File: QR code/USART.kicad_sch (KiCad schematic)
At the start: 26 parts, among them J1 ON_24, J5 ON_5_3, J7 Usart_debbag, U4 AM1SS-2403SJZ, U4 AM1SS-2405SJZ, U5 Pai122E30

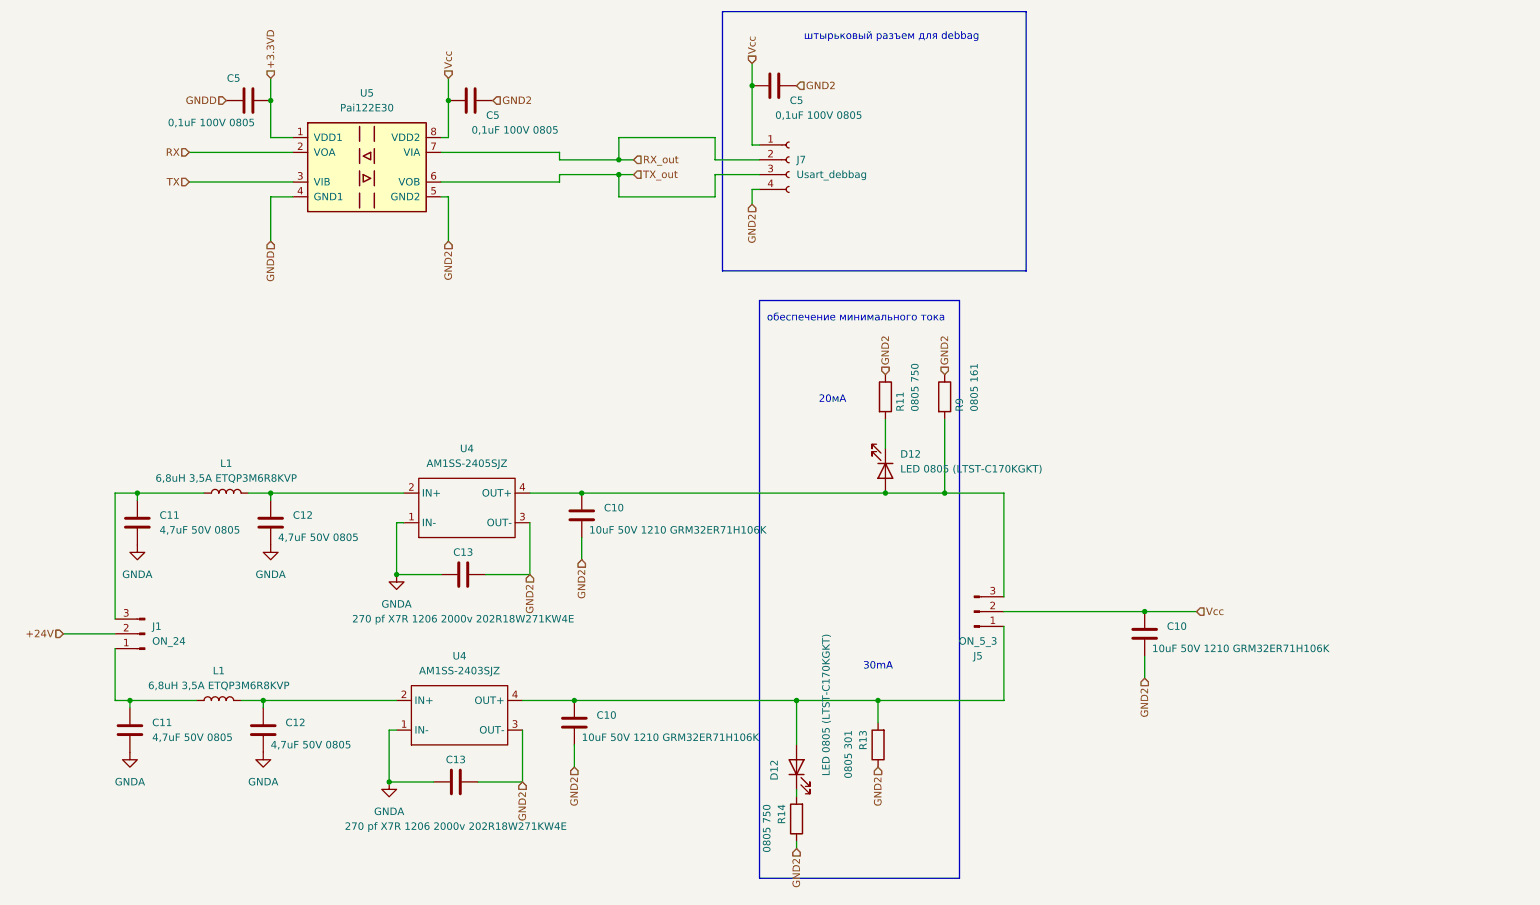
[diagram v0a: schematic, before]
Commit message: qr code schems
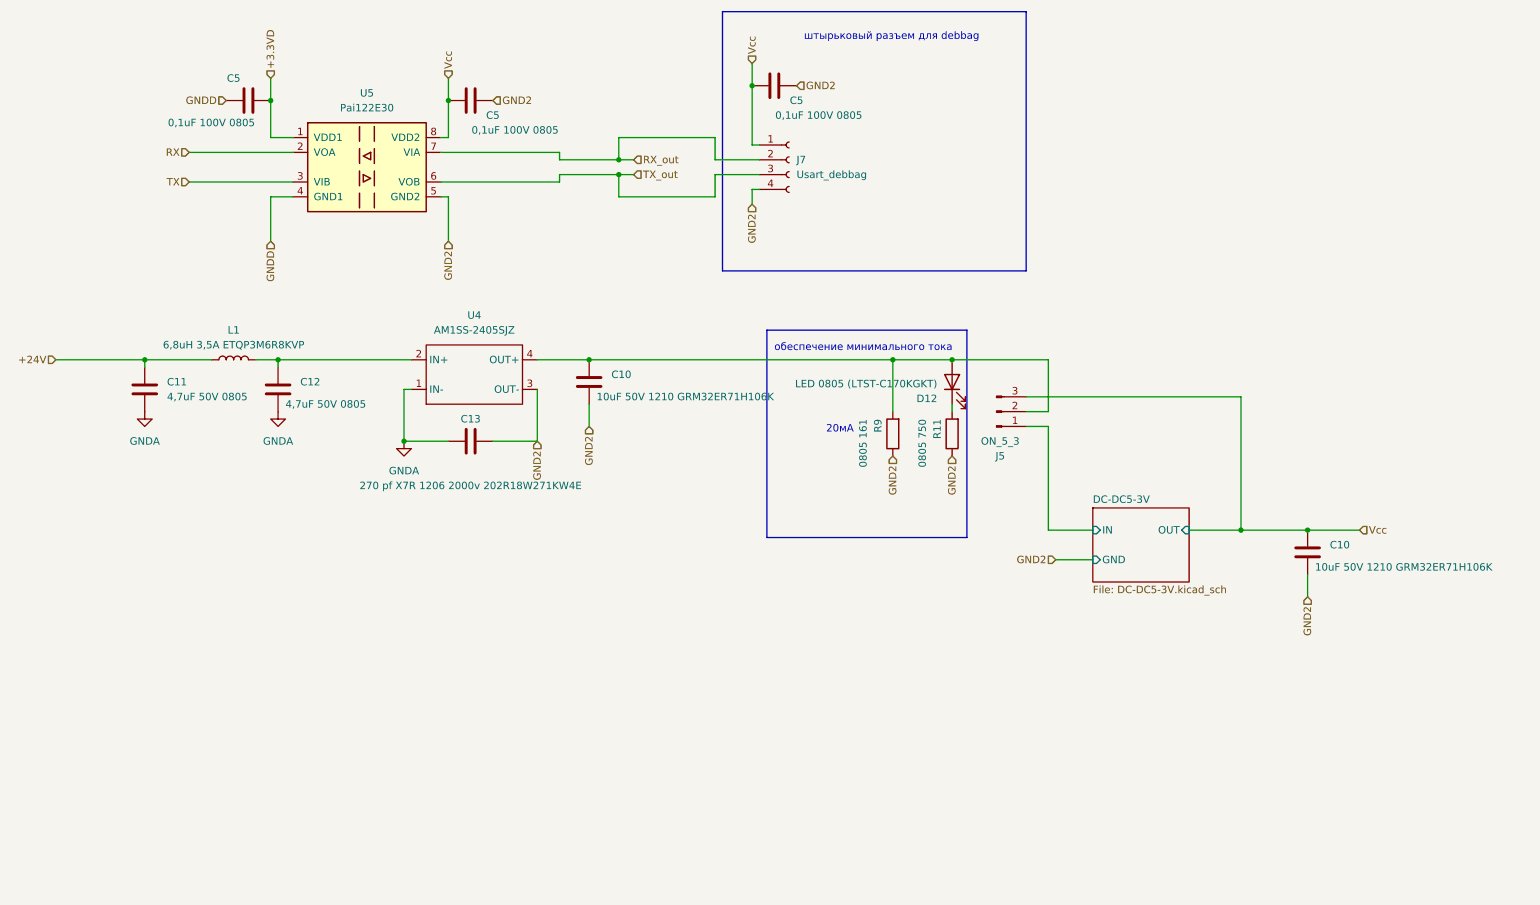
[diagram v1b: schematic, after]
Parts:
- removed C10: 10uF 50V 1210 GRM32ER71H106K, PCM_Capacitor_SMD_AKL:C_1210_3225Metric_Pad1.42x2.65mm_HandSolder, symbol Device:C
- removed C11, C12: 4,7uF 50V 0805, PCM_Capacitor_SMD_AKL:C_0805_2012Metric_Pad1.18x1.45mm_HandSolder, symbol Device:C
- removed C13: 270 pf X7R 1206 2000v 202R18W271KW4E, PCM_Capacitor_SMD_Handsoldering_AKL:C_1210_3225Metric_Pad1.42x2.65mm, symbol Device:C
- removed D12: LED 0805 (LTST-C170KGKT), LED_SMD:LED_0805_2012Metric_Pad1.15x1.40mm_HandSolder, symbol Device:LED
- removed J1: ON_24, Connector_PinHeader_2.54mm:PinHeader_1x03_P2.54mm_Vertical, symbol Connector:Conn_01x03_Pin
- removed L1: 6,8uH 3,5A ETQP3M6R8KVP, PCM_Inductor_SMD_Handsoldering_AKL:L_Bourns-SRN6028, symbol Device:L
- removed R13: 0805 301, Resistor_SMD:R_0805_2012Metric_Pad1.20x1.40mm_HandSolder, symbol Device:R
- removed R14: 0805 750, Resistor_SMD:R_0805_2012Metric_Pad1.20x1.40mm_HandSolder, symbol Device:R
- removed U4: AM1SS-2403SJZ, Converter_DCDC:Converter_DCDC_Murata_MEE3SxxxxSC_THT, symbol Converter_DCDC:AM1SS-
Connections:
- net +24V: now also C11.1, L1.1
- net Vcc: now also J5.3 (Pin_3); no longer J5.2 (Pin_2)
- net DC-DC5-3V/IN: now reaches J5.1 (Pin_1)
- net at C10.1, D12.2 (A), R9.2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: now also J5.2 (Pin_2); no longer J5.3 (Pin_3)
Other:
- added sheet DC-DC5-3V (DC-DC5-3V.kicad_sch)
- note removed: "30mA"
- moved on the sheet: C10, C11, C12, C13, D12, J5, L1, R11, R9, U4
